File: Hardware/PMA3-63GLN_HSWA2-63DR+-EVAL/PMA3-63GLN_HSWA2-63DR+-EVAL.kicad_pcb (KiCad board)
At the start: 2 copper layers, 32 x 48 mm, 19 parts, among them IC1 PMA3-63GLN+, IC2 PE42423B-Z, J1 Conn_Coaxial, J2 Conn_Coaxial, J3 Conn_Coaxial, J4 Conn_Coaxial, J5 Conn_Coaxial, J6 Conn_Coaxial, J7 Conn_Coaxial, J8 Conn_01x03_Pin, J9 Conn_01x03_Pin

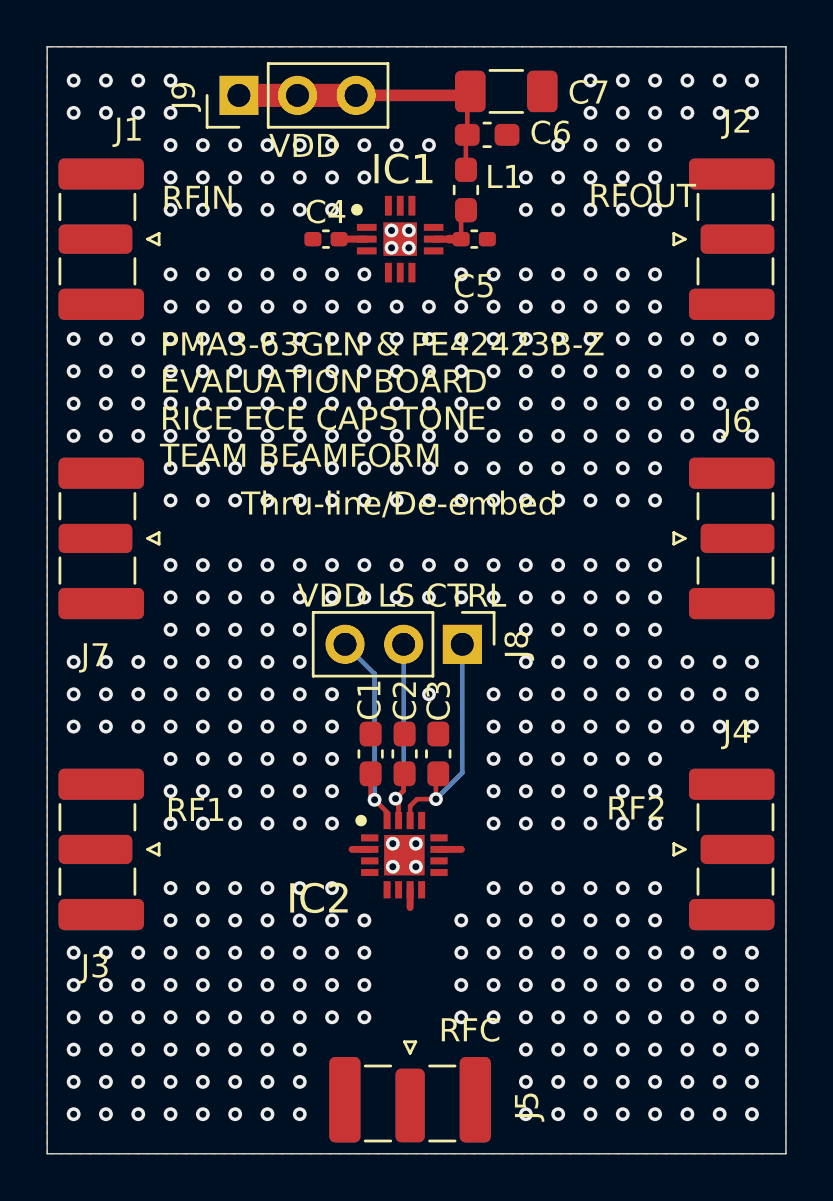
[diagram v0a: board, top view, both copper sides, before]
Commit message: EVAL board design files
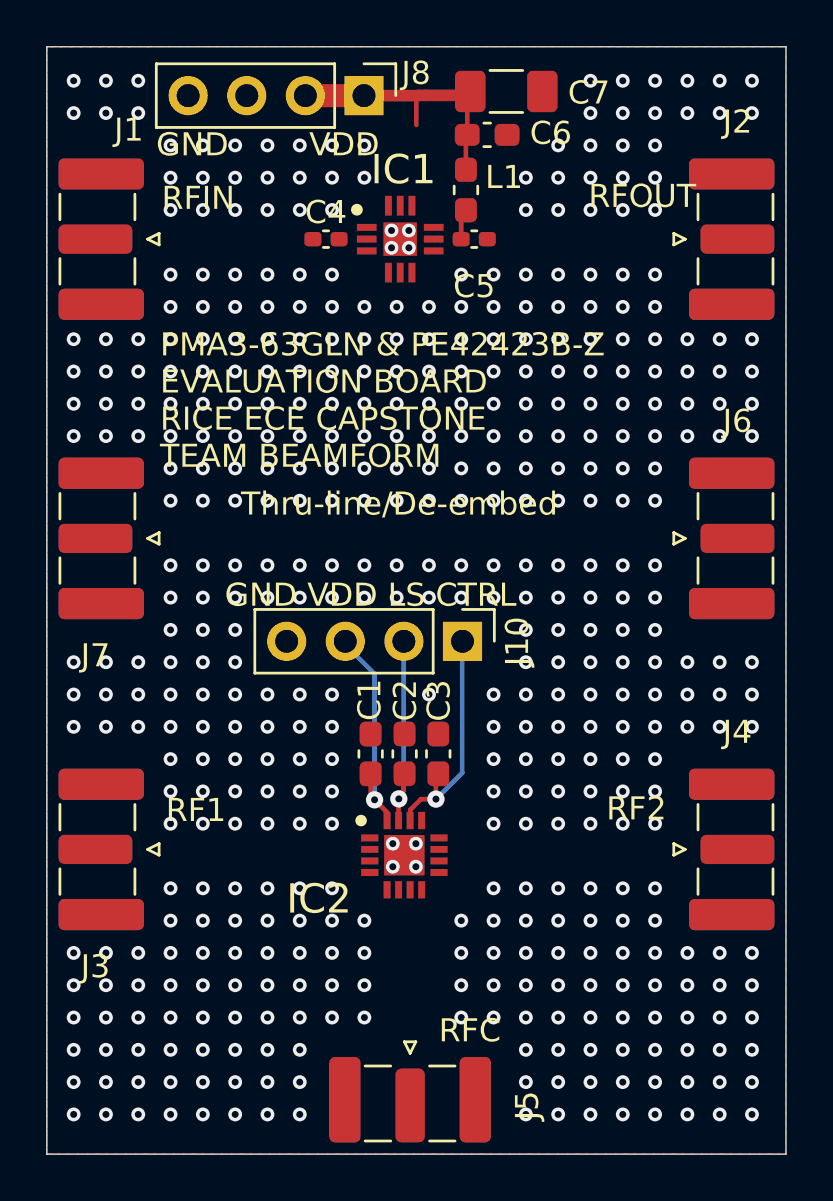
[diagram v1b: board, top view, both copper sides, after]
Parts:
- removed J9: Conn_01x03_Pin, Connector_PinHeader_2.54mm:PinHeader_1x03_P2.54mm_Vertical
- added J10: Conn_01x04_Pin, Connector_PinHeader_2.54mm:PinHeader_1x04_P2.54mm_Vertical, F.Cu at (101.6, 64.2)
- J8: value Conn_01x03_Pin -> Conn_01x04_Pin; footprint Connector_PinHeader_2.54mm:PinHeader_1x03_P2.54mm_Vertical -> Connector_PinHeader_2.54mm:PinHeader_1x04_P2.54mm_Vertical
- moved J8 24.2 mm to (97.3, 40.5)
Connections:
- J8 pad 1: CTRL -> VDD
- J8 pad 2: LS -> VDD
- J8 pad 3: VDD -> GND
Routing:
- net VDD: track 23.2 -> 21.6 mm
- net GND: vias 479 -> 470
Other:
- board text added: "GND VDD"
- board text added: "GND VDD LS CTRL"
- board text removed: "VDD"
- board text removed: "VDD LS CTRL"
